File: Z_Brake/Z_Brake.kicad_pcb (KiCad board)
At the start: 2 copper layers, 55.9 x 35.6 mm, 26 parts, among them K1 EC2-24NU, K2 EC2-24NU, P1 CONN_01X04, P2 CONN_01X02, P3 CONN_01X04, Q1 2N7002, U1 LM397

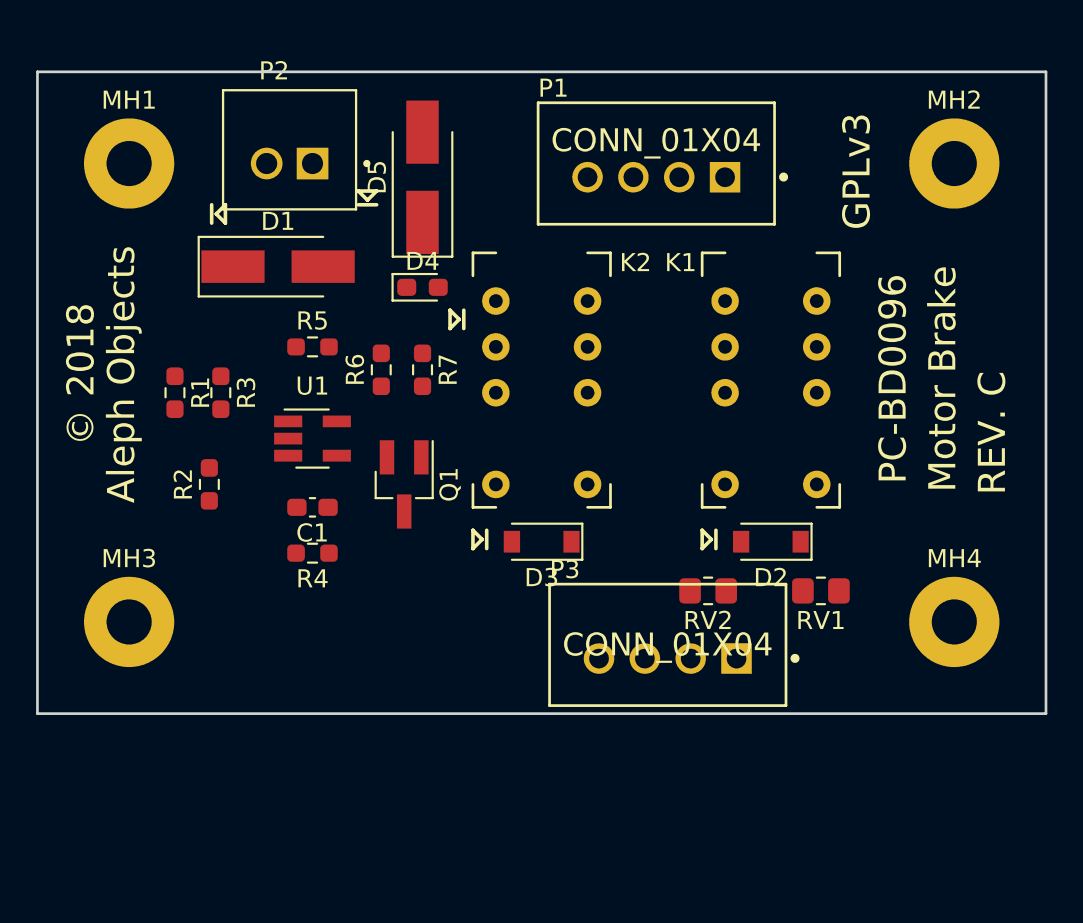
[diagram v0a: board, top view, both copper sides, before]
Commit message: Final PCB
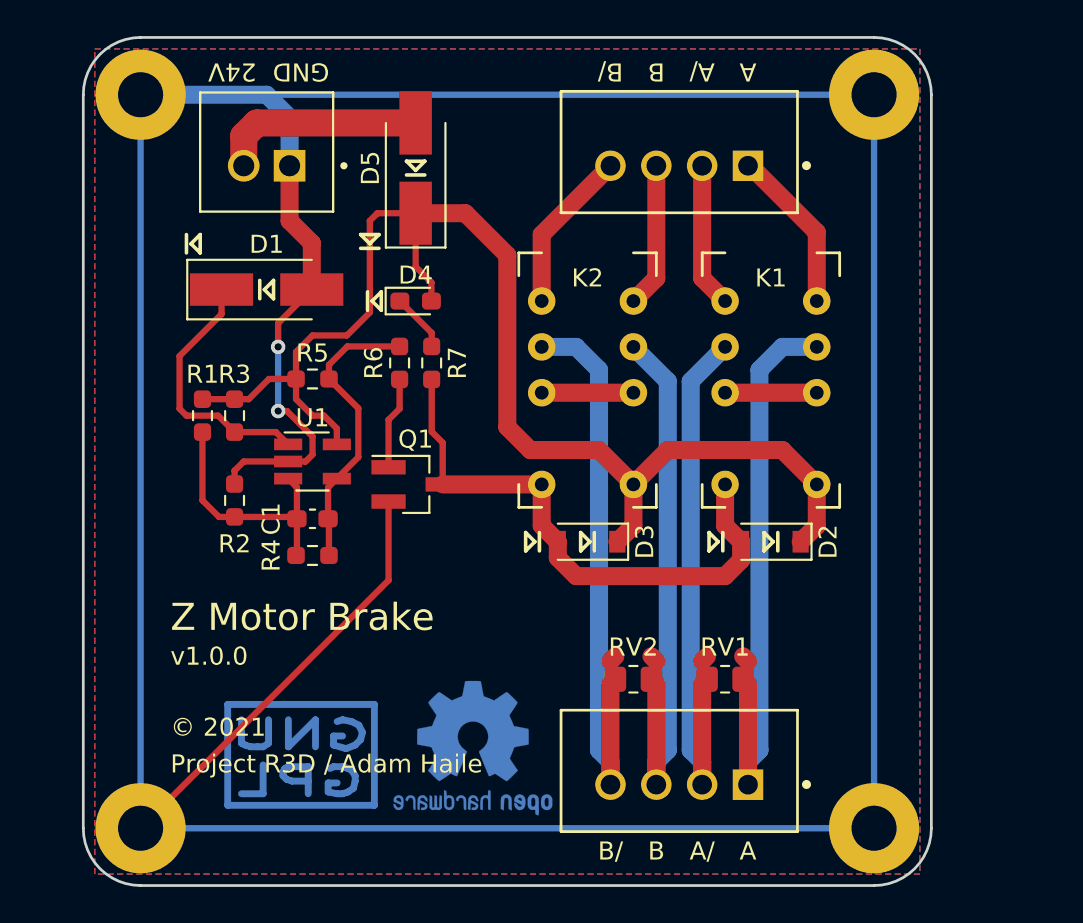
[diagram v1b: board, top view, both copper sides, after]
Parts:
- added REF**: Symbol_GNU-GPL_CopperTop_Small, Symbol:Symbol_GNU-GPL_CopperTop_Small, B.Cu at (67.9, 116.8)
- added REF**: OSHW-Logo2_9.8x8mm_Copper, Symbol:OSHW-Logo2_9.8x8mm_Copper, B.Cu at (77.5, 116.2)
- moved MH4 12.3 mm to (99.7, 120.7)
- moved MH3 11.4 mm to (59.1, 120.7)
- moved RV1 7.22 mm to (91.4, 112.4)
- moved P3 7.01 mm to (88.9, 117.5)
- moved RV2 6.41 mm to (86.4, 112.4)
- moved MH2 5.85 mm to (99.7, 80.0)
- moved MH1 3.86 mm to (59.1, 80.0)
- moved D3 2.54 mm to (83.8, 104.8)
- moved K2 2.54 mm to (83.8, 96.5)
- moved R1 1.98 mm to (62.5, 97.8)
- moved R5 1.78 mm to (68.6, 95.8)
- moved R2 1.66 mm to (64.3, 102.5)
- moved R3 1.48 mm to (64.3, 97.8)
- moved D1 1.42 mm to (66.0, 90.8)
- moved P1 1.42 mm to (88.9, 83.2)
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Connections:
- D4 pad 1: VDD -> Net-(D4-Pad1)
- D4 pad 2: Net-(D4-Pad2) -> VDD
- R7 pad 1: Net-(D4-Pad2) -> Net-(D4-Pad1)
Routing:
- net GND: track 0.00 -> 221.6 mm, vias 0 -> 2
- net VDD: track 0.00 -> 72.8 mm
- net Net-(K2-Pad9): track 0.00 -> 32.9 mm
- net Net-(K1-Pad4): track 0.00 -> 32.9 mm
- net Net-(D2-Pad2): track 0.00 -> 31.5 mm
- net Net-(K2-Pad4): track 0.00 -> 31.3 mm
- net Net-(K1-Pad9): track 0.00 -> 31.3 mm
- net Net-(C1-Pad1): track 0.00 -> 16.3 mm
- net Net-(D1-Pad1): track 0.00 -> 14.4 mm
- net Net-(C1-Pad2): track 0.00 -> 13.9 mm
- net +24V: track 0.00 -> 11.5 mm
- net Net-(K1-Pad5): track 0.00 -> 9.15 mm
- net Net-(K2-Pad8): track 0.00 -> 9.07 mm
- net Net-(K2-Pad5): track 0.00 -> 8.02 mm
- net Net-(K1-Pad8): track 0.00 -> 8.02 mm
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- added copper zone on B.Cu, net GND
- added copper zone on F.Cu, net GND
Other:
- board size 55.9 x 35.6 mm -> 47 x 47 mm
- net class Default: trace_width 0.381 -> 0.25; via_dia 1.016 -> 1.2; via_drill 0.508 -> 0.6
- net class STD_Signal removed
- net class VDD added: clearance 0.2, trace_width 1, via_dia 1.6, via_drill 0.8
- rule via_min_drill: 0.508 -> 0.4
- rule via_min_size: 1.016 -> 0.8
- board text added: "24V"
- board text added: "A"
- board text added: "A/"
- board text added: "B"
- board text added: "B/"
- board text added: "GND"
- board text added: "Original 2 motor design by Aleph Objects 2018"
- board text added: "Project R3D / Adam Haile"
- board text added: "Z Motor Brake"
- board text added: "v1.0.0"
- board text added: "© 2021"
- board text removed: "Aleph Objects"
- board text removed: "GPLv3"
- board text removed: "Motor Brake"
- board text removed: "PC-BD0096"
- board text removed: "REV. C"
- board text removed: "© 2018"
